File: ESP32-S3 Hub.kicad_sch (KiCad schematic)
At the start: 23 parts, among them U1 ESP32-S3, Y1 ABM11-40.000MHZ-B1U-T3, 10ppm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

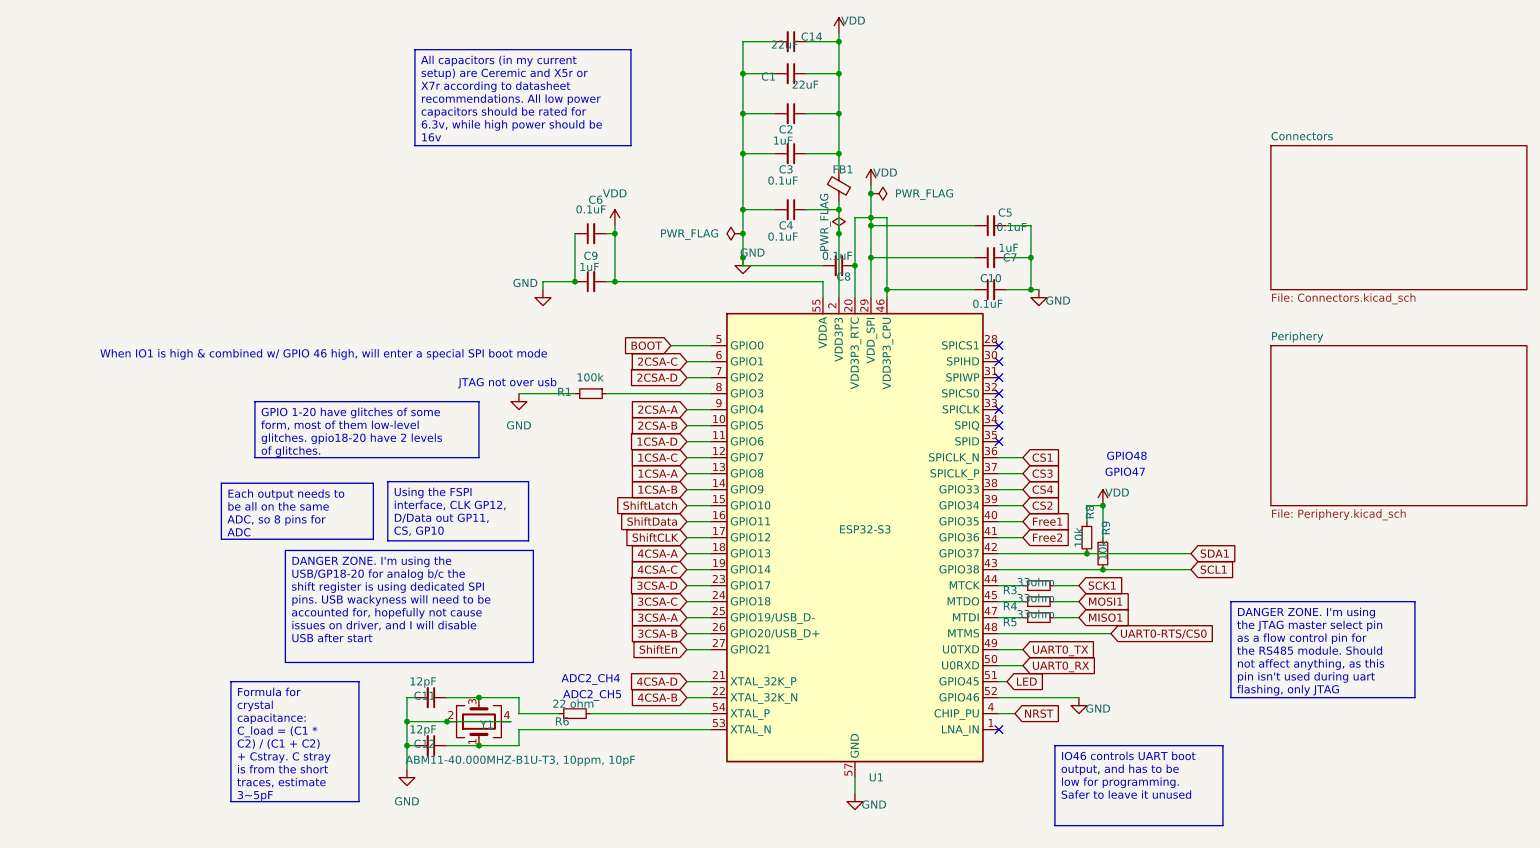
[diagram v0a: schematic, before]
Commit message: Improve schematic consistency
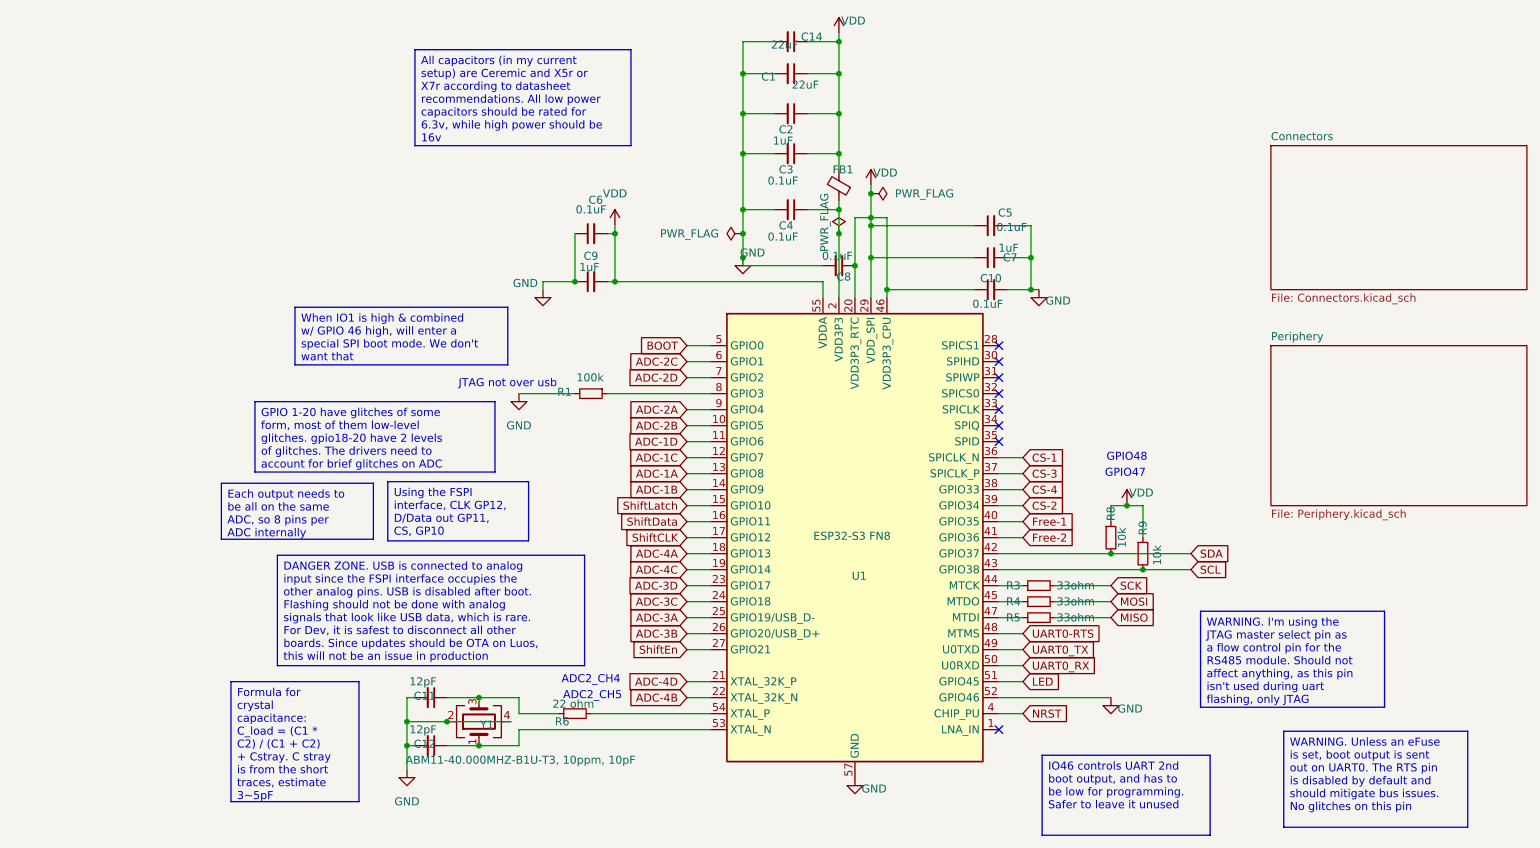
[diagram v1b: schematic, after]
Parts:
- U1: value ESP32-S3 -> ESP32-S3 FN8
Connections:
- net 1CSA-A renamed ADC-1A
- net 1CSA-B renamed ADC-1B
- net 1CSA-C renamed ADC-1C
- net 1CSA-D renamed ADC-1D
- net 2CSA-A renamed ADC-2A
- net 2CSA-B renamed ADC-2B
- net 2CSA-C renamed ADC-2C
- net 2CSA-D renamed ADC-2D
- net 3CSA-A renamed ADC-3A
- net 3CSA-B renamed ADC-3B
- net 3CSA-C renamed ADC-3C
- net 3CSA-D renamed ADC-3D
- net 4CSA-A renamed ADC-4A
- net 4CSA-B renamed ADC-4B
- net 4CSA-C renamed ADC-4C
- net 4CSA-D renamed ADC-4D
- net CS1 renamed CS-1
- net CS2 renamed CS-2
- net CS3 renamed CS-3
- net CS4 renamed CS-4
- net Free1 renamed Free-1
- net Free2 renamed Free-2
- net MISO1 renamed MISO
- net MOSI1 renamed MOSI
- net SCK1 renamed SCK
- net SCL1 renamed SCL
- net SDA1 renamed SDA
- net UART0-RTS/CS0 renamed UART0-RTS
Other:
- note removed: "When IO1 is high & combined w/ GPIO 46 high, will enter a special SPI boot mode"
- moved on the sheet: R8, R9
